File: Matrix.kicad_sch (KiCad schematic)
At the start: 2 parts

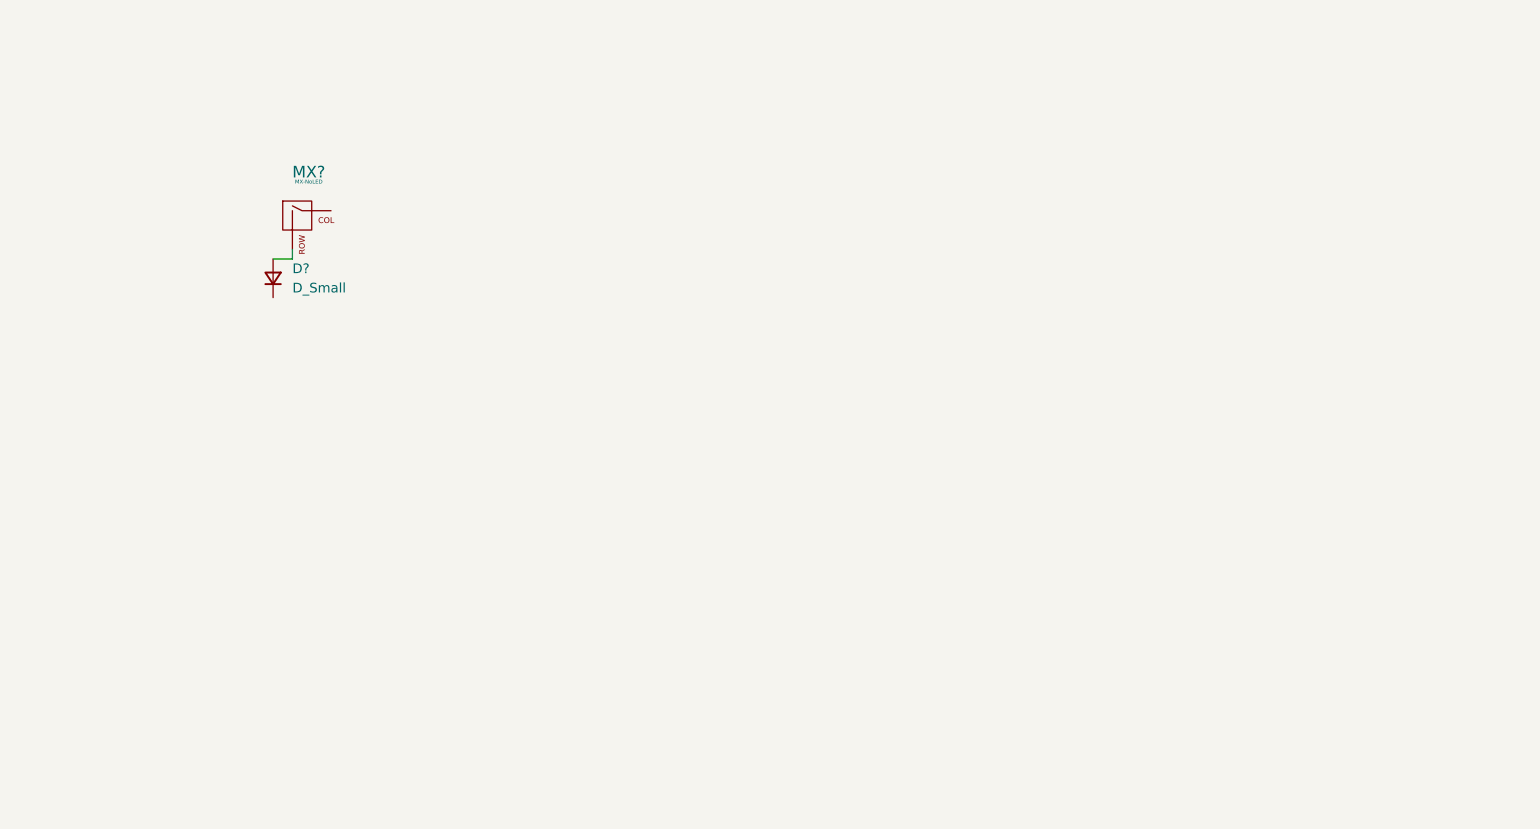
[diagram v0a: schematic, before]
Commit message: matrix done
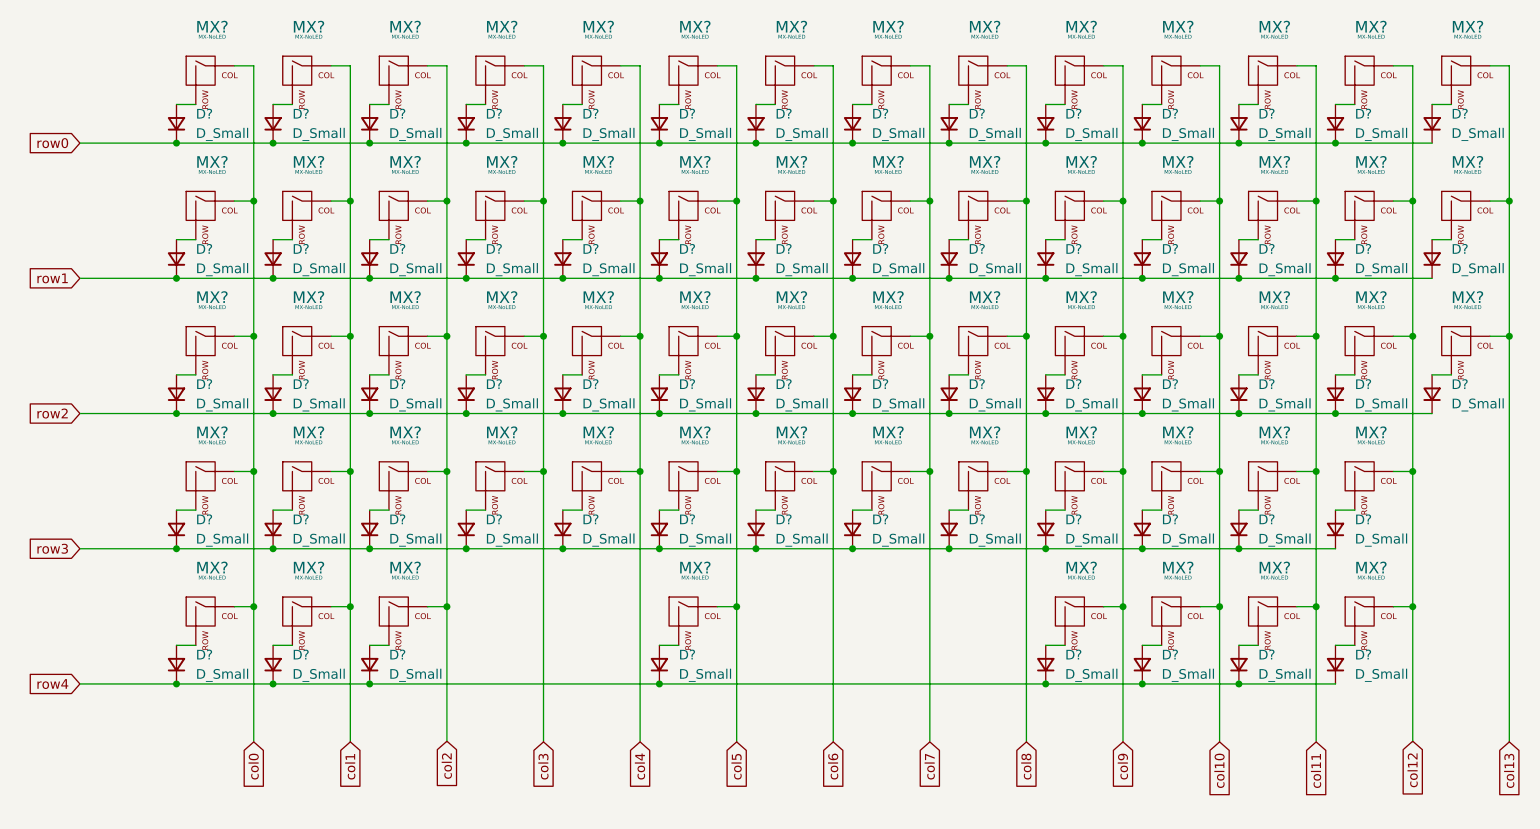
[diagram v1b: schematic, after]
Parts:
- added D? (x62): D_Small, symbol Device:D_Small
- added MX? (x62): MX-NoLED, symbol MX_Alps_Hybrid:MX-NoLED
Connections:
- net col0: now reaches MX?.1 (COL)
- net col0: now also MX?.1 (COL), MX?.1 (COL), MX?.1 (COL), MX?.1 (COL)
- net row0: now reaches D?.1 (K)
- net row0: now also D?.1 (K), D?.1 (K), D?.1 (K), D?.1 (K), D?.1 (K), D?.1 (K), D?.1 (K), D?.1 (K), D?.1 (K), D?.1 (K), D?.1 (K), D?.1 (K), D?.1 (K)
- new net: D?.2 (A), MX?.2 (ROW) (x62)
- new net col1: MX?.1 (COL), MX?.1 (COL), MX?.1 (COL), MX?.1 (COL), MX?.1 (COL)
- new net col10: MX?.1 (COL), MX?.1 (COL), MX?.1 (COL), MX?.1 (COL), MX?.1 (COL)
- new net col11: MX?.1 (COL), MX?.1 (COL), MX?.1 (COL), MX?.1 (COL), MX?.1 (COL)
- new net col12: MX?.1 (COL), MX?.1 (COL), MX?.1 (COL), MX?.1 (COL), MX?.1 (COL)
- new net col13: MX?.1 (COL), MX?.1 (COL), MX?.1 (COL)
- new net col2: MX?.1 (COL), MX?.1 (COL), MX?.1 (COL), MX?.1 (COL), MX?.1 (COL)
- new net col3: MX?.1 (COL), MX?.1 (COL), MX?.1 (COL), MX?.1 (COL)
- new net col4: MX?.1 (COL), MX?.1 (COL), MX?.1 (COL), MX?.1 (COL)
- new net col5: MX?.1 (COL), MX?.1 (COL), MX?.1 (COL), MX?.1 (COL), MX?.1 (COL)
- new net col6: MX?.1 (COL), MX?.1 (COL), MX?.1 (COL), MX?.1 (COL)
- new net col7: MX?.1 (COL), MX?.1 (COL), MX?.1 (COL), MX?.1 (COL)
- new net col8: MX?.1 (COL), MX?.1 (COL), MX?.1 (COL), MX?.1 (COL)
- new net col9: MX?.1 (COL), MX?.1 (COL), MX?.1 (COL), MX?.1 (COL), MX?.1 (COL)
- new net row1: D?.1 (K), D?.1 (K), D?.1 (K), D?.1 (K), D?.1 (K), D?.1 (K), D?.1 (K), D?.1 (K), D?.1 (K), D?.1 (K), D?.1 (K), D?.1 (K), D?.1 (K), D?.1 (K)
- new net row2: D?.1 (K), D?.1 (K), D?.1 (K), D?.1 (K), D?.1 (K), D?.1 (K), D?.1 (K), D?.1 (K), D?.1 (K), D?.1 (K), D?.1 (K), D?.1 (K), D?.1 (K), D?.1 (K)
- new net row3: D?.1 (K), D?.1 (K), D?.1 (K), D?.1 (K), D?.1 (K), D?.1 (K), D?.1 (K), D?.1 (K), D?.1 (K), D?.1 (K), D?.1 (K), D?.1 (K), D?.1 (K)
- new net row4: D?.1 (K), D?.1 (K), D?.1 (K), D?.1 (K), D?.1 (K), D?.1 (K), D?.1 (K), D?.1 (K)
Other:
- moved on the sheet: D?, MX?
